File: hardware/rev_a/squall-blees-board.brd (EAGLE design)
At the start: 48.3 x 50.2 mm, 7 parts, among them J1 SQUALL_HEADER, J4 HIROSE-DF40C-10DP-0.4V, J5 HIROSE-DF40C-10DP-0.4V

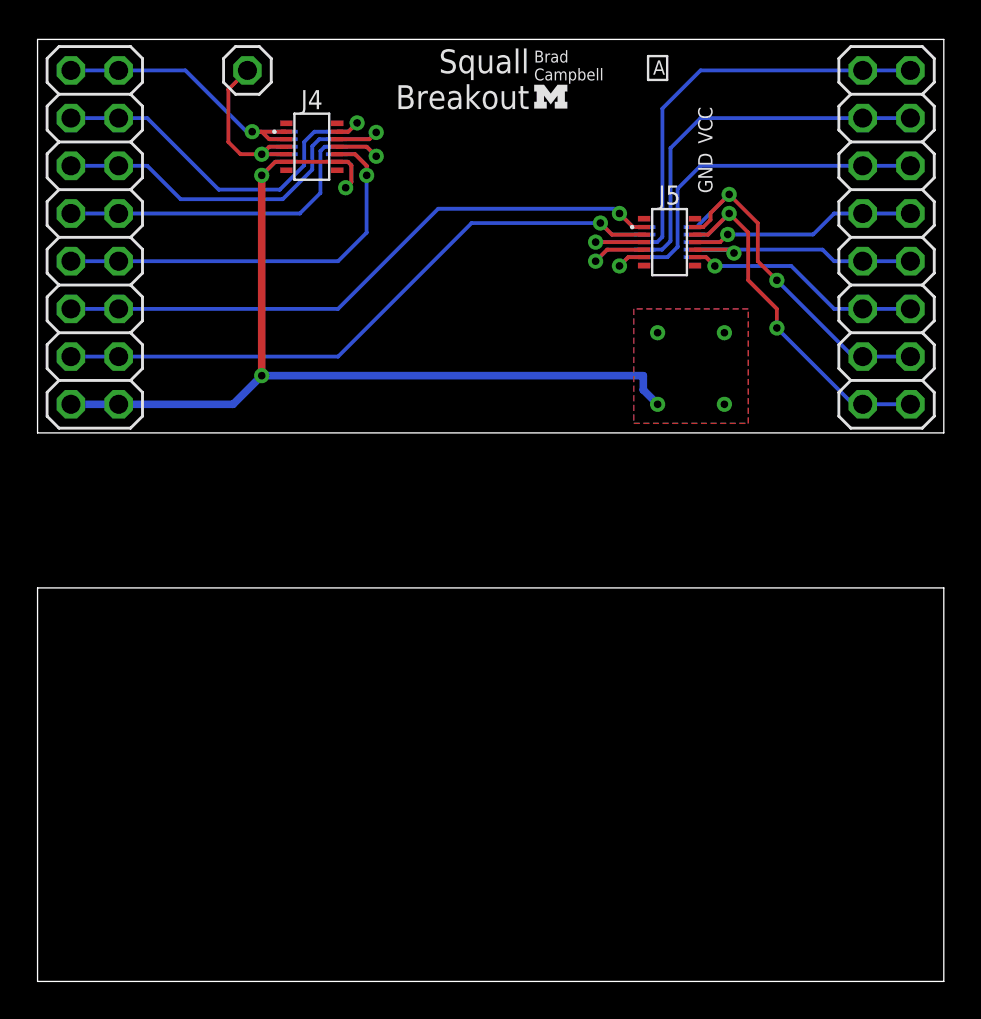
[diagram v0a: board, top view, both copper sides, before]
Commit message: Work on circuit board
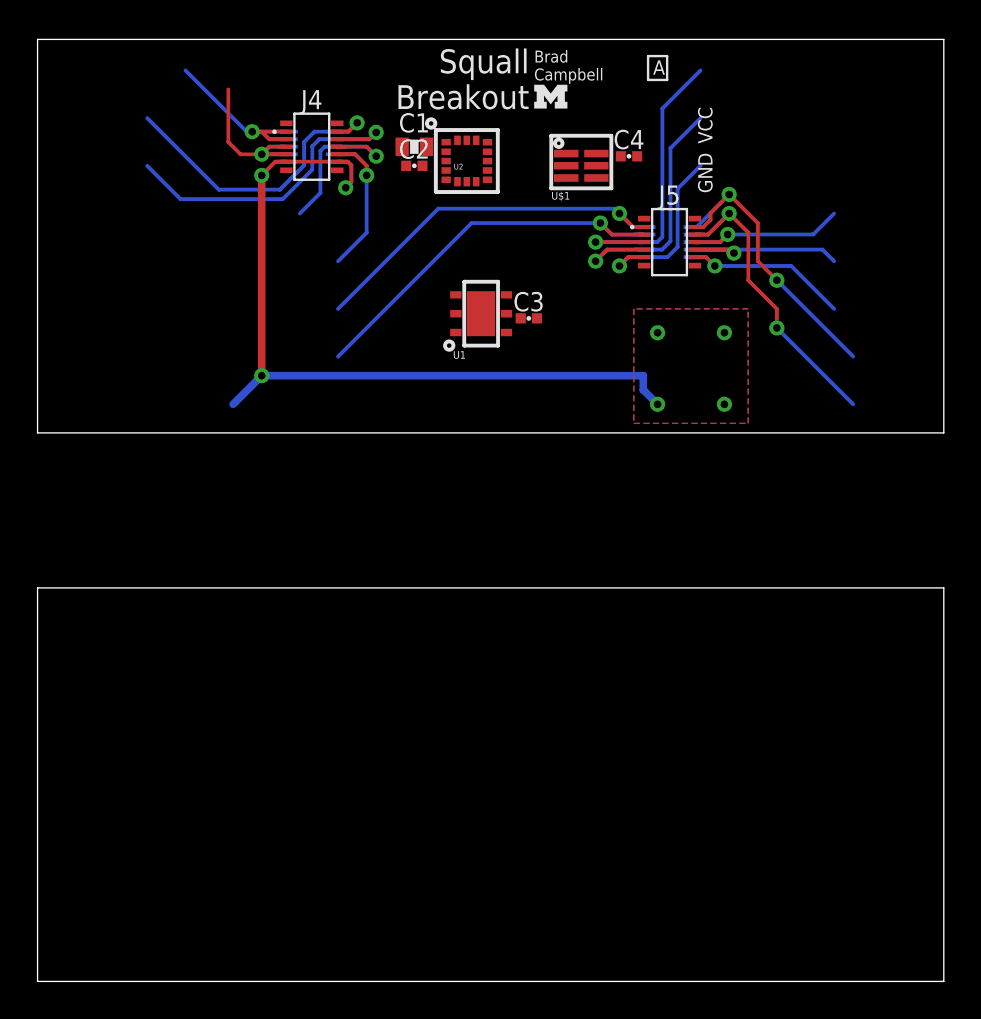
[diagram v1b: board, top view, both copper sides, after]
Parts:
- removed J2, J3: (no value), pinhead:2X08
- removed J6: (no value), pinhead:1X01
- added C1: 10uF, passives:0603_CAP
- added C2, C3, C4: 100nF, passives:0402_CAP
- added U$1: TSL2560DFN, blees:DFN2
- added U1: HTU21DDFN, blees:DFN
- added U2: LPS331APQFN, blees:HCLGA-16L
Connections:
- net 5V: no longer J6.1
- net A5: no longer J3.5, J3.6
- net A6: no longer J3.3, J3.4
- net A7: no longer J3.1, J3.2
- net GND: now also C1.2, C2.2, C3.2, C4.2, U$1.2, U$1.3, U1.2, U1.PAD, U2.10, U2.12, U2.13, U2.16, U2.5, U2.7; no longer J2.15, J2.16
- net MISO: no longer J3.10, J3.9
- net MOSI: no longer J3.7, J3.8
- net P22: no longer J2.3, J2.4
- net P23: no longer J2.5, J2.6
- net P24: no longer J2.7, J2.8
- net P25: no longer J2.10, J2.9
- net SCL: now also U$1.4, U1.6, U2.4; no longer J2.13, J2.14
- net SCLK: no longer J3.11, J3.12
- net SDA: now also U$1.6, U1.1, U2.6; no longer J2.11, J2.12
- net SWDCLK: no longer J3.13, J3.14
- net SWDIO/!RESET: no longer J3.15, J3.16
- net VCC: now also C1.1, C2.1, C3.1, C4.1, U$1.1, U1.5, U2.1, U2.14, U2.15, U2.8; no longer J2.1, J2.2
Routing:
- net P25: track 24.1 -> 9.90 mm
- net SDA: track 34.8 -> 20.6 mm
- net SCL: track 36.3 -> 22.1 mm
- net P24: track 21.5 -> 9.34 mm
- net A6: track 25.7 -> 14.5 mm
- net A7: track 27.1 -> 16.0 mm
- net A5: track 21.0 -> 9.85 mm
- net GND: track 53.9 -> 45.3 mm
- net VCC: track 18.2 -> 12.1 mm
- net P23: track 21.4 -> 17.4 mm
- net P22: track 20.3 -> 16.2 mm
- net MOSI: track 14.1 -> 9.99 mm
- net MISO: track 16.1 -> 12.0 mm
- net SCLK: track 13.9 -> 9.84 mm
- net SWDIO/!RESET: track 20.5 -> 17.5 mm
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
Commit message: Board finished
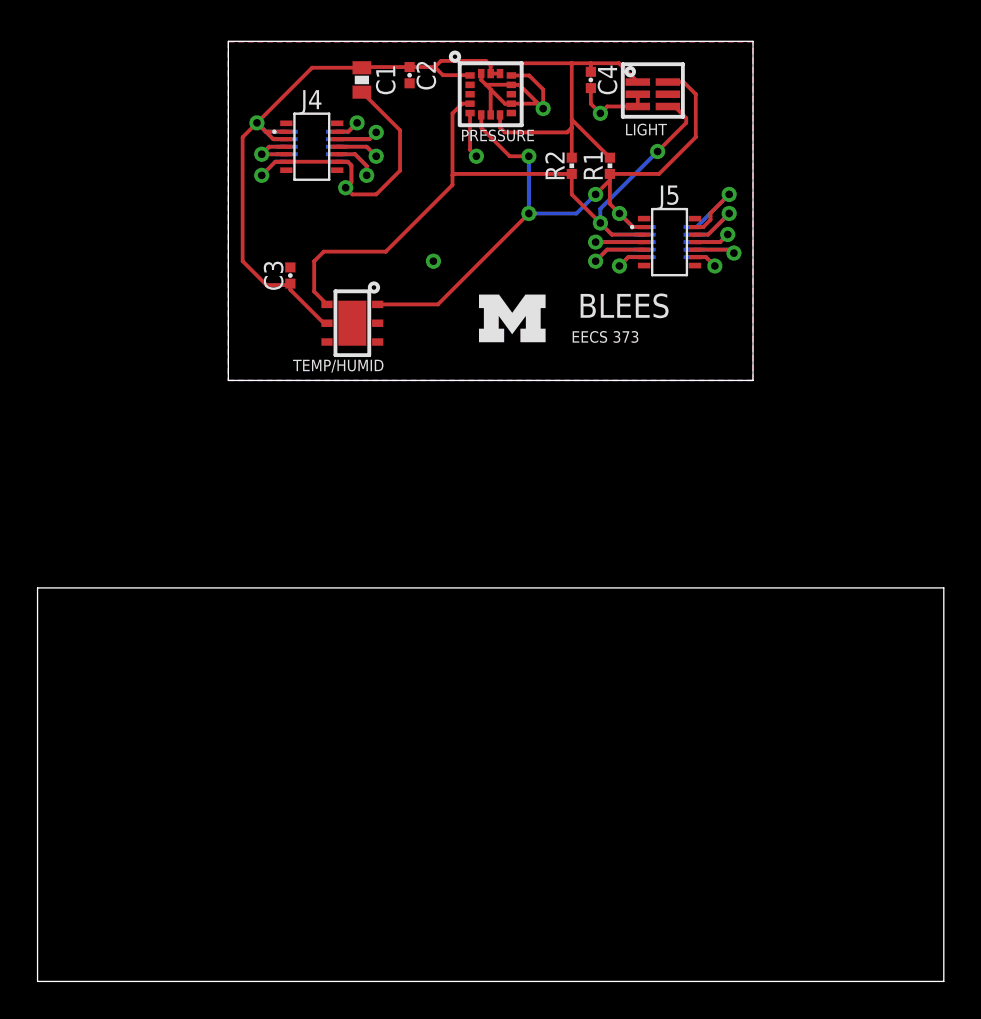
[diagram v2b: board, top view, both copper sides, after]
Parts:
- removed LOGO1: UMICH_SOLID_TINY, logos:UMICH_SOLID_50MIL
- removed U$1: TSL2560DFN, blees:DFN2
- removed U1: HTU21DDFN, blees:DFN
- removed U2: LPS331APQFN, blees:HCLGA-16L
- added LIGHT: TSL2560DFN, blees:DFN2
- added PRESSURE: LPS331APQFN, blees:HCLGA-16L
- added R1, R2: 2kΩ, passives:0402_RES
- added TEMP/HUMID: HTU21DDFN, blees:DFN
- moved C3 12.9 mm to (13.5, 8.38), turned to 90 degrees
- moved C2 4.83 mm to (19.8, 19.1), turned to 270 degrees
- moved C4 4.54 mm to (29.5, 18.8), turned to 270 degrees
- moved C1 4.52 mm to (17.3, 18.8), turned to 270 degrees
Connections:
- net GND: now also LIGHT.2, LIGHT.3, PRESSURE.10, PRESSURE.12, PRESSURE.13, PRESSURE.16, PRESSURE.5, PRESSURE.7, TEMP/HUMID.2, TEMP/HUMID.PAD; no longer U$1.2, U$1.3, U1.2, U1.PAD, U2.10, U2.12, U2.13, U2.16, U2.5, U2.7
- net SCL: now also LIGHT.4, PRESSURE.4, R2.1, TEMP/HUMID.6; no longer U$1.4, U1.6, U2.4
- net SDA: now also LIGHT.6, PRESSURE.6, R1.1, TEMP/HUMID.1; no longer U$1.6, U1.1, U2.6
- net VCC: now also LIGHT.1, PRESSURE.1, PRESSURE.14, PRESSURE.15, PRESSURE.8, R1.2, R2.2, TEMP/HUMID.5; no longer U$1.1, U1.5, U2.1, U2.14, U2.15, U2.8
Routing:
- net VCC: track 12.1 -> 58.9 mm
- net SCL: track 22.1 -> 40.1 mm, vias 1 -> 2
- net SDA: track 20.6 -> 37.7 mm, vias 1 -> 4
- net P22: track 16.2 -> 2.54 mm
- net SWDIO/!RESET: track 17.5 -> 4.61 mm, vias 2 -> 1
- net P23: track 17.4 -> 4.48 mm
- net SWDCLK: track 16.7 -> 5.32 mm, vias 2 -> 1
- net A7: track 16.0 -> 5.20 mm
- net A6: track 14.5 -> 5.71 mm
- net MISO: track 12.0 -> 4.34 mm
- net GND: track 45.3 -> 37.9 mm, vias 7 -> 6
- net SCLK: track 9.84 -> 2.54 mm
- net A5: track 9.85 -> 3.05 mm
- net MOSI: track 9.99 -> 3.86 mm
- net P25: track 9.90 -> 4.69 mm
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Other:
- board size 48.3 x 50.2 mm -> 48.3 x 50.1 mm
- board text added: "BLEES"
- board text added: "EECS 373"
- board text removed: "3V3"
- board text removed: "5V"
- board text removed: "A"
- board text removed: "A5"
- board text removed: "A6"
- board text removed: "A7"
- board text removed: "Brad Campbell"
- board text removed: "GND"
- board text removed: "MISO"
- board text removed: "MOSI"
- board text removed: "P22"
- board text removed: "P23"
- board text removed: "P24"
- board text removed: "P25"
- board text removed: "SCL"
- board text removed: "SCLK"
- board text removed: "SDA"
- board text removed: "SWDC"
- board text removed: "SWDI"
- board text removed: "Squall Breakout"
- board text removed: "VCC"

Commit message: Board ready for prod
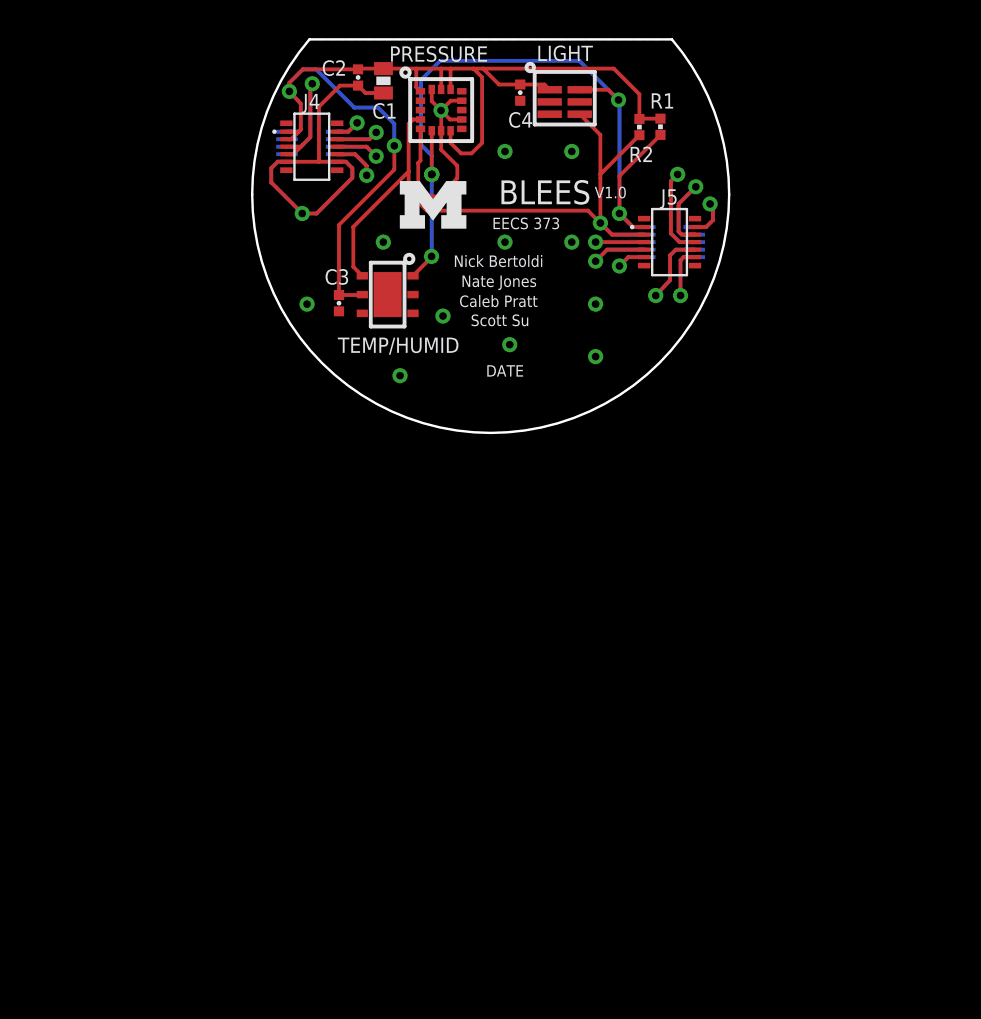
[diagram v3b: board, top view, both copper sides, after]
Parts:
- moved LIGHT 4.71 mm to (28.1, 17.6)
- moved R2 4.15 mm to (32.0, 16.3)
- moved C4 3.82 mm to (25.7, 18.1)
- moved R1 3.40 mm to (33.2, 16.3)
- moved C3 2.98 mm to (16.1, 6.91), turned to 270 degrees
- moved PRESSURE 2.77 mm to (21.5, 17.2)
- moved C2 2.75 mm to (17.1, 18.9)
- moved TEMP/HUMID 2.42 mm to (18.6, 7.37)
- moved C1 1.15 mm to (18.4, 18.8)
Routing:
- net MOSI: track 3.86 -> 9.50 mm
- net 5V: track 5.65 -> 10.6 mm
- net VCC: track 58.9 -> 63.8 mm, vias 1 -> 2
- net SDA: track 37.7 -> 42.0 mm, vias 4 -> 5
- net SCL: track 40.1 -> 36.6 mm, vias 2 -> 1
- net GND: track 37.9 -> 41.4 mm, vias 6 -> 12
- net MISO: track 4.34 -> 7.75 mm
- net SCLK: track 2.54 -> 5.40 mm
- net SWDIO/!RESET: track 4.61 -> 7.37 mm
- net SWDCLK: track 5.32 -> 4.11 mm
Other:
- board size 48.3 x 50.1 mm -> 25.4 x 21 mm
- board text added: "Caleb Pratt"
- board text added: "DATE"
- board text added: "Nate Jones"
- board text added: "Nick Bertoldi"
- board text added: "Scott Su"
- board text added: "V1.0"
